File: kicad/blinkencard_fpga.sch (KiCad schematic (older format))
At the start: 18 parts, among them U1 ICE40UP5K-SG48ITR, U2 W25Q64JV

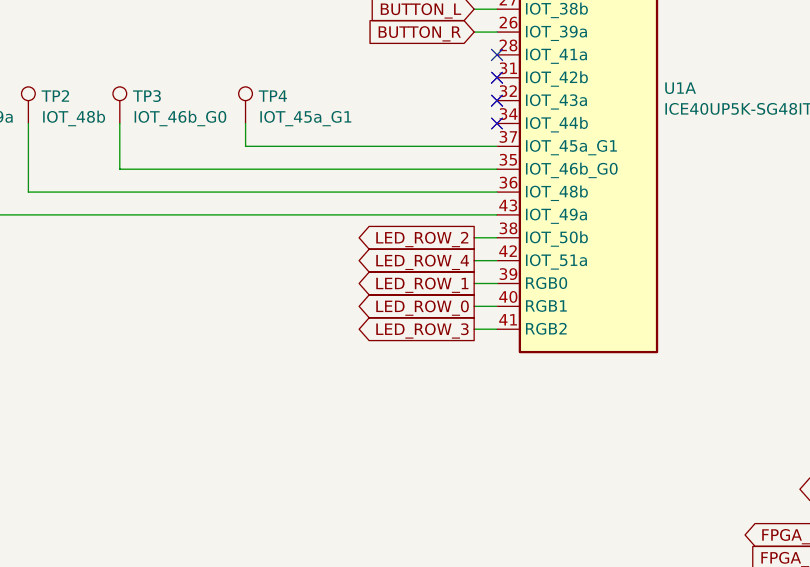
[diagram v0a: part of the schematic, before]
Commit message: LED routing
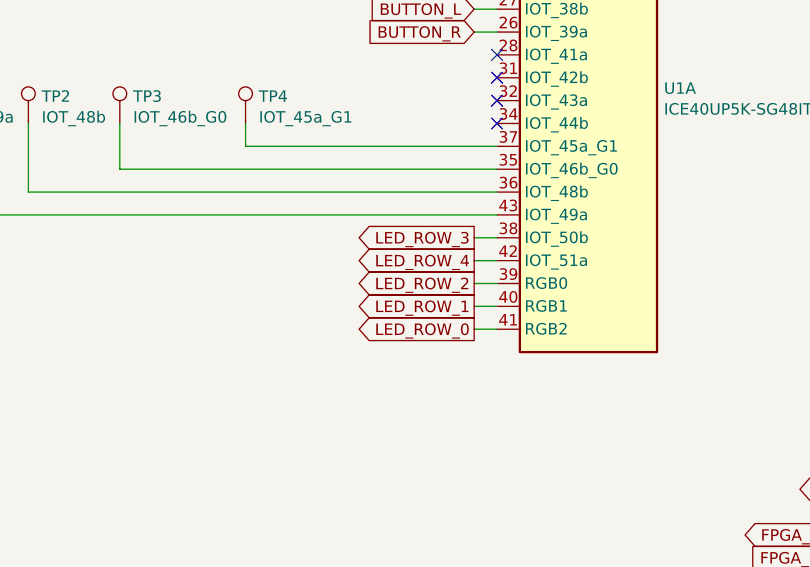
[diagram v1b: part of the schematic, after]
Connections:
- net LED_ROW_0: now also U1.41 (RGB2); no longer U1.40 (RGB1)
- net LED_ROW_1: now also U1.40 (RGB1); no longer U1.39 (RGB0)
- net LED_ROW_2: now also U1.39 (RGB0); no longer U1.38 (IOT_50b)
- net LED_ROW_3: now also U1.38 (IOT_50b); no longer U1.41 (RGB2)
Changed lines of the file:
@@
 	1    0    0    -1
 $EndComp
-Text GLabel 2900 3500 0    50   Output ~ 0
+Text GLabel 2900 3600 0    50   Output ~ 0
 LED_ROW_0
 Text GLabel 2900 3400 0    50   Output ~ 0
-LED_ROW_1
+LED_ROW_2
 Text GLabel 2900 3200 0    50   Output ~ 0
-LED_ROW_2
-Text GLabel 2900 3600 0    50   Output ~ 0
 LED_ROW_3
-Text GLabel 2900 3300 0    50   Output ~ 0
-LED_ROW_4
 Wire Wire Line
 	3000 3200 2900 3200
@@
 	1    0    0    -1
 $EndComp
+Text GLabel 2900 3500 0    50   Output ~ 0
+LED_ROW_1
+Text GLabel 2900 3300 0    50   Output ~ 0
+LED_ROW_4
 $EndSCHEMATC
